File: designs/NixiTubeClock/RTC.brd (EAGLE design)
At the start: 160 x 100 mm, 7 parts, among them IC1 DS1307N+, U1 S8411-45R, Y1 CM7V-T1A-32.768K-9PF-20PPM-TA-

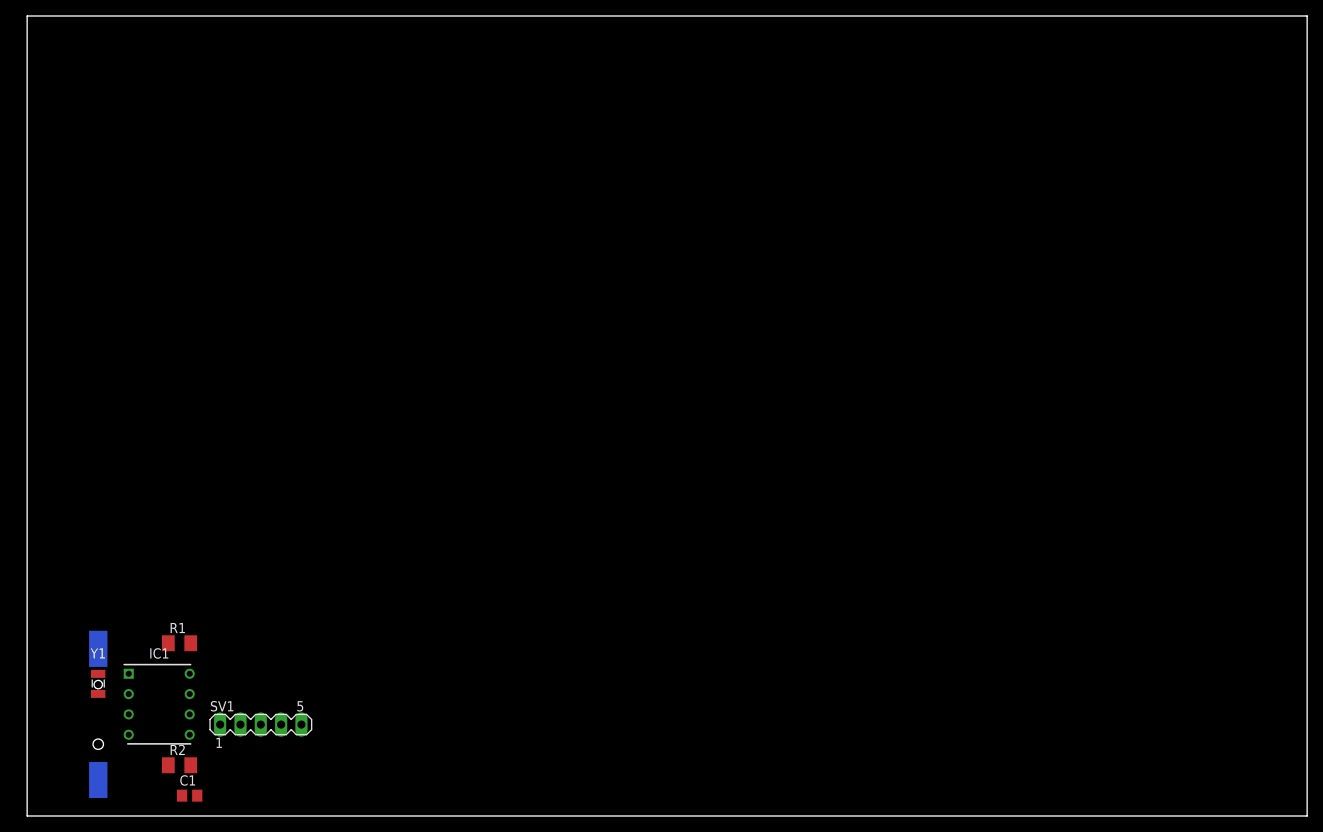
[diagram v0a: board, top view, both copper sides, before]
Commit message: updated RTC BRD
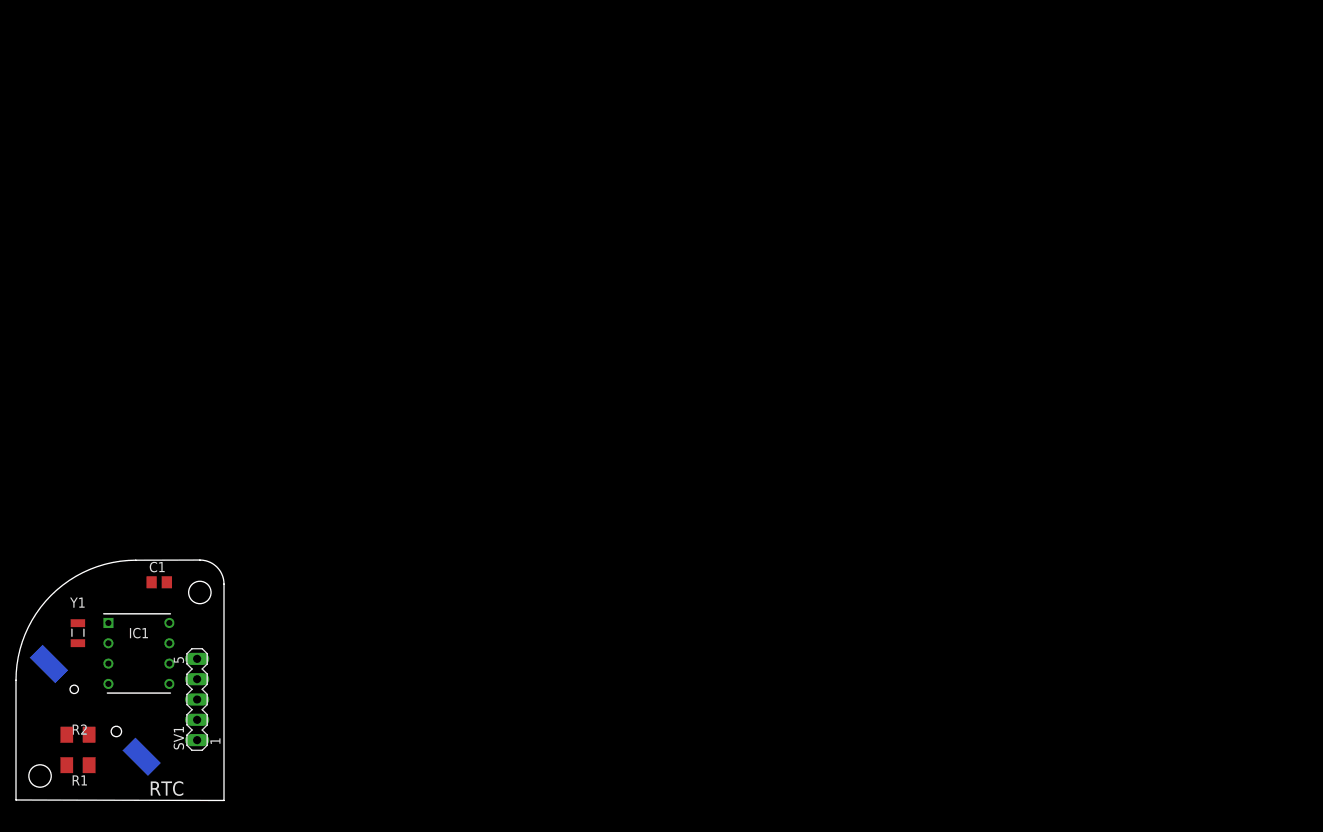
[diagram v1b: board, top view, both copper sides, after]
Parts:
- moved C1 26.9 mm to (16.5, 29.2)
- moved R1 19.8 mm to (6.35, 6.35), turned to 180 degrees
- moved R2 13.3 mm to (6.35, 10.2), turned to 180 degrees
- moved SV1 8.55 mm to (21.2, 14.6), turned to 90 degrees
- moved IC1 6.84 mm to (14.0, 20.3)
- moved Y1 6.84 mm to (6.35, 22.9)
- moved U1 0.62 mm to (8.52, 13.2), turned to 315 degrees
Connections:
- net SCL: now also SV1.2; no longer SV1.3
- net SDA: now also SV1.3; no longer SV1.4
- net SQW/OUT: now also SV1.1; no longer SV1.2
- net VCC: now also SV1.4; no longer SV1.1
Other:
- board size 160 x 100 mm -> 26 x 30.1 mm
- board text added: "RTC"
